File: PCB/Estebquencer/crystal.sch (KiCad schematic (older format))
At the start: 3 parts

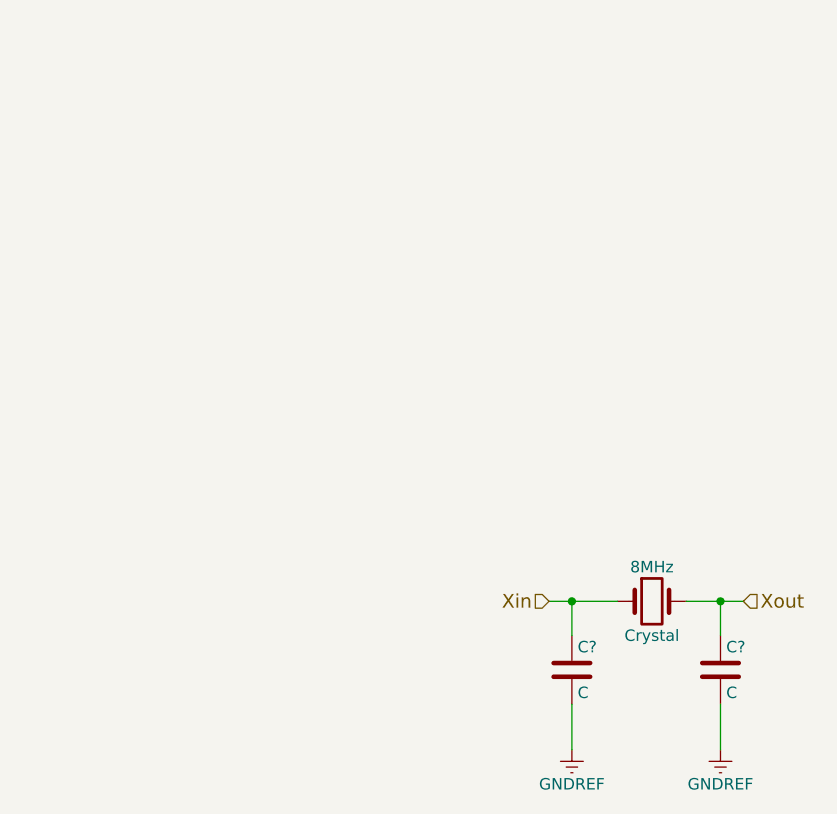
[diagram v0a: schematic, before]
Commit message: acabado módulo ARM
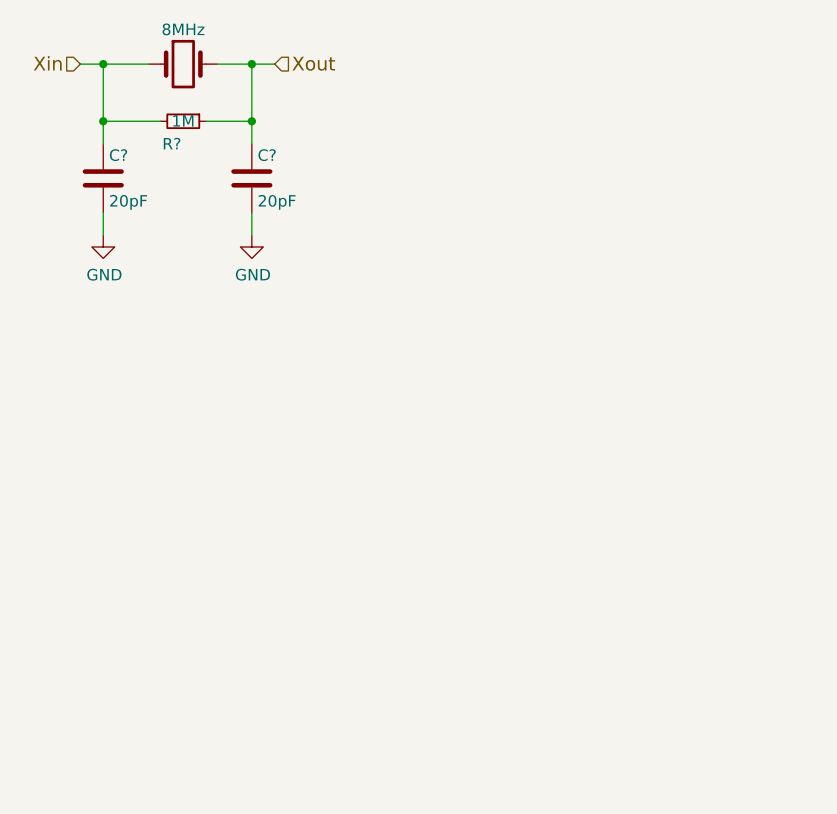
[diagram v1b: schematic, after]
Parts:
- removed C?: C, symbol Estebquencer-rescue:C
- added C?: 20pF, symbol Estebquencer-rescue:C
- added R?: 1M, symbol Device:R_Small
- C?: value C -> 20pF
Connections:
- net Xin: now also R?.2
- net Xout: now also C?.1, R?.1
- net GNDREF renamed GND
- net GND: now also C?.2
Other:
- moved on the sheet: 8MHz, C?
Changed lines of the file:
@@
 EELAYER 26 0
 EELAYER END
-$Descr A4 11693 8268
+$Descr User 5906 4000
 encoding utf-8
-Sheet 8 10
+Sheet 7 10
 Title ""
 Date ""
@@
 L Estebquencer-rescue:Crystal 8MHz
 U 1 1 5875B883
-P 4950 3400
-F 0 "8MHz" H 4950 3550 50  0000 C CNN
-F 1 "Crystal" H 4950 3250 50  0000 C CNN
-F 2 "" H 4950 3400 50  0000 C CNN
-F 3 "" H 4950 3400 50  0000 C CNN
-	1    4950 3400
+P 2900 1050
+F 0 "8MHz" H 2900 1200 50  0000 C CNN
+F 1 "Crystal" H 2900 1050 50  0001 C CNN
+F 2 "" H 2900 1050 50  0000 C CNN
+F 3 "" H 2900 1050 50  0000 C CNN
+	1    2900 1050
 	1    0    0    -1
 $EndComp
@@
 L Estebquencer-rescue:C C?
 U 1 1 5875B8B9
-P 4600 3700
-F 0 "C?" H 4625 3800 50  0000 L CNN
-F 1 "C" H 4625 3600 50  0000 L CNN
-F 2 "" H 4638 3550 50  0000 C CNN
-F 3 "" H 4600 3700 50  0000 C CNN
-	1    4600 3700
+P 2550 1550
+F 0 "C?" H 2575 1650 50  0000 L CNN
+F 1 "20pF" H 2575 1450 50  0000 L CNN
+F 2 "" H 2588 1400 50  0000 C CNN
+F 3 "" H 2550 1550 50  0000 C CNN
+	1    2550 1550
+	1    0    0    -1
+$EndComp
+Wire Wire Line
+	2450 1050 2550 1050
+Wire Wire Line
+	3050 1050 3200 1050
+Text HLabel 2450 1050 0    60   Input ~ 0
+Xin
+Text HLabel 3300 1050 2    60   Input ~ 0
+Xout
+Connection ~ 3200 1050
+Connection ~ 2550 1050
+Wire Wire Line
+	3200 1050 3300 1050
+Wire Wire Line
+	2550 1050 2750 1050
+$Comp
+L power:GND #PWR?
+U 1 1 5E3C8828
+P 2550 1800
+F 0 "#PWR?" H 2550 1550 50  0001 C CNN
+F 1 "GND" H 2555 1627 50  0000 C CNN
+F 2 "" H 2550 1800 50  0001 C CNN
+F 3 "" H 2550 1800 50  0001 C CNN
+	1    2550 1800
+	1    0    0    -1
+$EndComp
+$Comp
+L power:GND #PWR?
+U 1 1 5E3C885B
+P 3200 1800
+F 0 "#PWR?" H 3200 1550 50  0001 C CNN
+F 1 "GND" H 3205 1627 50  0000 C CNN
+F 2 "" H 3200 1800 50  0001 C CNN
+F 3 "" H 3200 1800 50  0001 C CNN
+	1    3200 1800
 	1    0    0    -1
 $EndComp
 $Comp
 L Estebquencer-rescue:C C?
-U 1 1 5875B8FC
-P 5250 3700
-F 0 "C?" H 5275 3800 50  0000 L CNN
-F 1 "C" H 5275 3600 50  0000 L CNN
-F 2 "" H 5288 3550 50  0000 C CNN
-F 3 "" H 5250 3700 50  0000 C CNN
-	1    5250 3700
-	1    0    0    -1
-$EndComp
-Wire Wire Line
-	4500 3400 4600 3400
-Wire Wire Line
-	4600 3400 4600 3550
-Wire Wire Line
-	5100 3400 5250 3400
-Wire Wire Line
-	5250 3400 5250 3550
-$Comp
-L power:GNDREF #PWR?
-U 1 1 5875B99F
-P 4600 4050
-F 0 "#PWR?" H 4600 3800 50  0001 C CNN
-F 1 "GNDREF" H 4600 3900 50  0000 C CNN
-F 2 "" H 4600 4050 50  0000 C CNN
-F 3 "" H 4600 4050 50  0000 C CNN
-	1    4600 4050
+U 1 1 5E3CA94D
+P 3200 1550
+F 0 "C?" H 3225 1650 50  0000 L CNN
+F 1 "20pF" H 3225 1450 50  0000 L CNN
+F 2 "" H 3238 1400 50  0000 C CNN
+F 3 "" H 3200 1550 50  0000 C CNN
+	1    3200 1550
 	1    0    0    -1
 $EndComp
 $Comp
-L power:GNDREF #PWR?
-U 1 1 5875B9BA
-P 5250 4050
-F 0 "#PWR?" H 5250 3800 50  0001 C CNN
-F 1 "GNDREF" H 5250 3900 50  0000 C CNN
-F 2 "" H 5250 4050 50  0000 C CNN
-F 3 "" H 5250 4050 50  0000 C CNN
-	1    5250 4050
-	1    0    0    -1
+L Device:R_Small R?
+U 1 1 5E3CAEF4
+P 2900 1300
+F 0 "R?" V 3000 1250 50  0000 C CNN
+F 1 "1M" V 2900 1300 50  0000 C CNN
+F 2 "" H 2900 1300 50  0001 C CNN
+F 3 "~" H 2900 1300 50  0001 C CNN
+	1    2900 1300
+	0    1    1    0
 $EndComp
 Wire Wire Line
-	5250 4050 5250 3850
+	2550 1050 2550 1300
 Wire Wire Line
-	4600 3850 4600 4050
-Text HLabel 4500 3400 0    60   Input ~ 0
-Xin
-Text HLabel 5350 3400 2    60   Input ~ 0
-Xout
-Connection ~ 5250 3400
-Connection ~ 4600 3400
+	2800 1300 2550 1300
+Connection ~ 2550 1300
 Wire Wire Line
-	5250 3400 5350 3400
+	2550 1300 2550 1400
 Wire Wire Line
-	4600 3400 4800 3400
+	3000 1300 3200 1300
+Wire Wire Line
+	3200 1050 3200 1300
+Wire Wire Line
+	3200 1400 3200 1300
+Connection ~ 3200 1300
+Wire Wire Line
+	3200 1700 3200 1800
+Wire Wire Line
+	2550 1800 2550 1700
 $EndSCHEMATC
